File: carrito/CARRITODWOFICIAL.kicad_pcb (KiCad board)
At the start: 2 copper layers, 155 x 92.3 mm, 113 parts, among them J10 MOTOR DE2, J11 LED2, J12 LED3, J13 foto, J14 IR, J15 LUZIZ, J16 LUZDE, J17 LBLUE2, J18 LRED2, J19 LRED1, J2 AUDIO, J20 LBLUE1, J21 servo 1, J22 servo 2, J23 servo 3, J24 Conn_01x15, J25 Conn_01x15, J4 MOTOR IZ1, J5 MOTOR IZ2, J6 Bocina, J7 BATERIA 12V, J8 LED1, J9 MOTOR DE1, Q1 2N3904, Q10 2N3904, Q11 IRF9540N, Q12 IRF3205, Q13 IRF3710, Q14 IRF3205, Q15 IRF9540N, Q16 IRF3205, Q17 2N3904, Q18 IRF3710, Q19 2N3904, Q2 IRF9540N, Q20 2N3904, Q21 2N3904, Q22 2N3904, Q23 2N3904, Q24 2N3904, Q25 2N3904, Q3 IRF3205, Q4 IRF3205, Q5 IRF9540N, Q6 IRF3205, Q7 IRF3205, Q8 2N3904, Q9 IRF3205, U1 PC817, U10 L7805, U2 PC817, U3 PC817, U4 L7805, U5 PC817, U6 L7805, U7 PC817, U8 PC817, U9 LM358

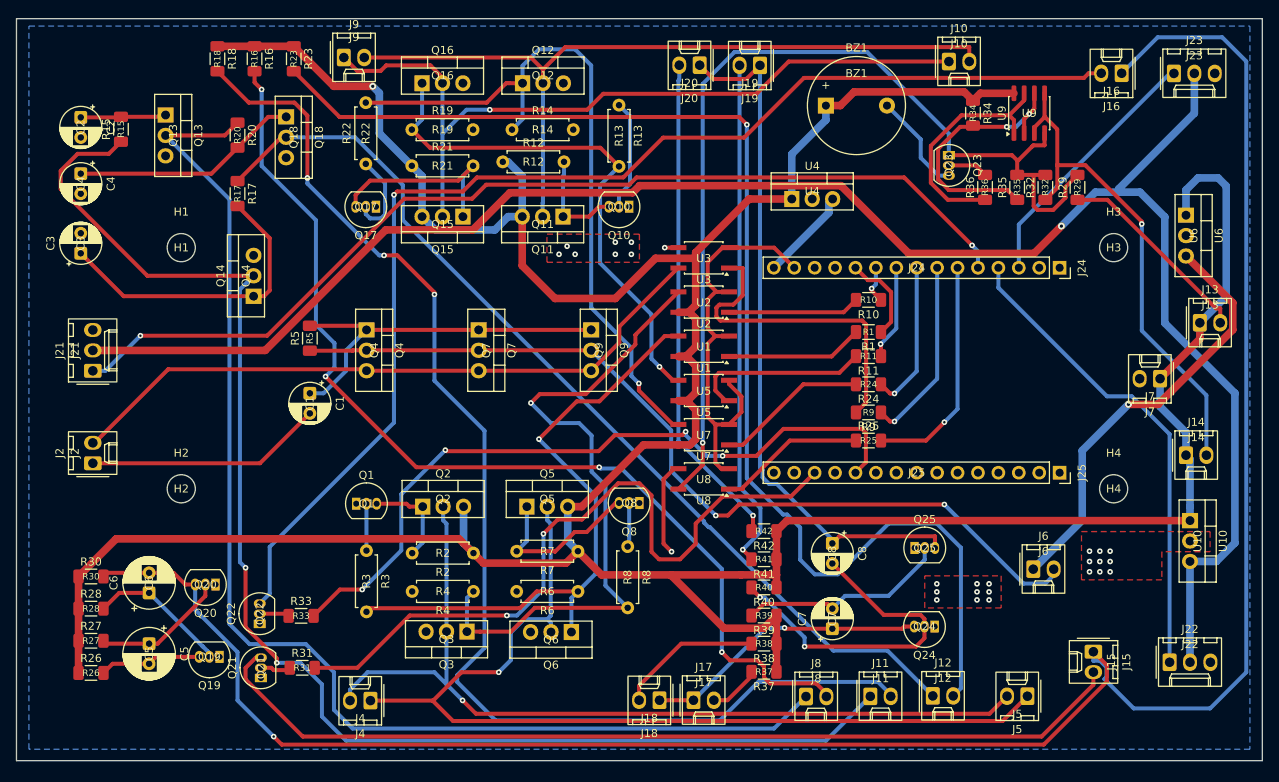
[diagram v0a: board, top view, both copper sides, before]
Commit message: Add files via upload
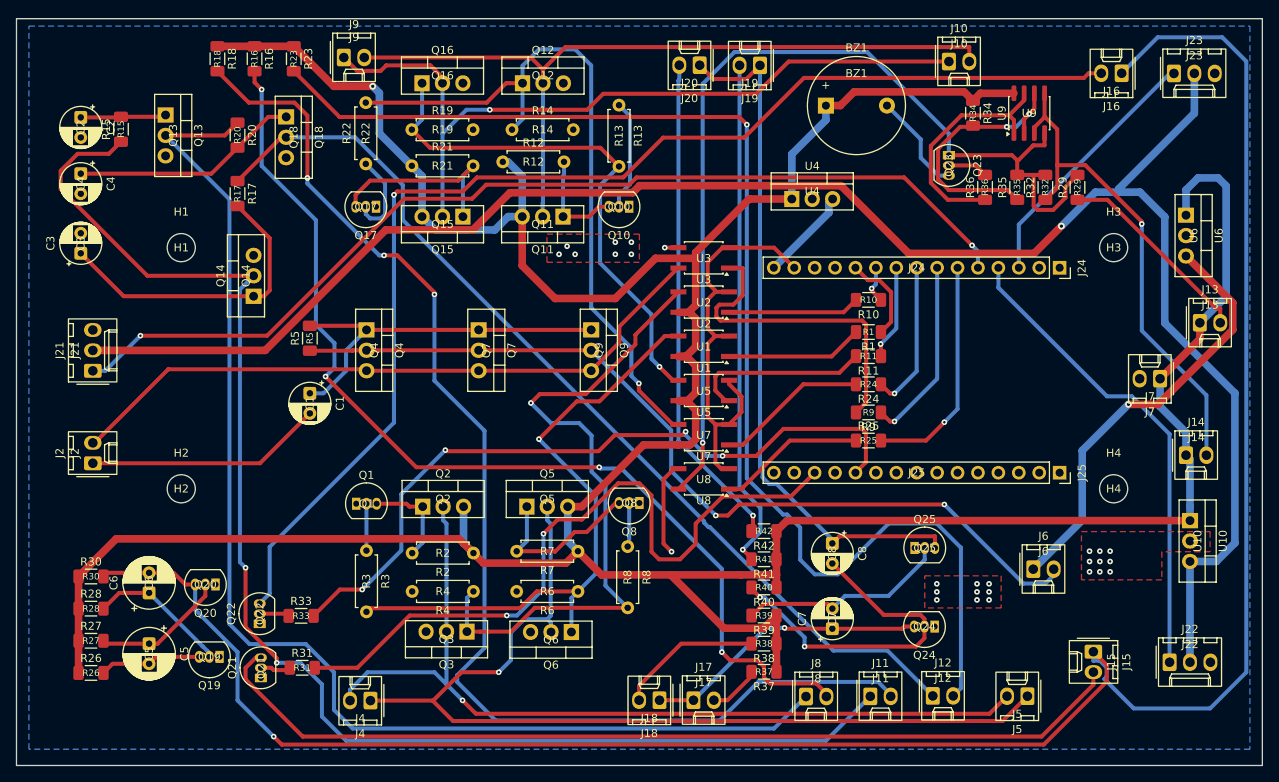
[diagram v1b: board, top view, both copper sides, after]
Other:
- board size 155 x 92.3 mm -> 155 x 92.9 mm
